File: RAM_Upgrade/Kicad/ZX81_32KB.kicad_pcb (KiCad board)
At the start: 2 copper layers, 23 x 44 mm, 3 parts, among them IC1 CY62256NLL-55SNXI, J3 Conn_01x04_Pin, J4 828-AG11D-LF

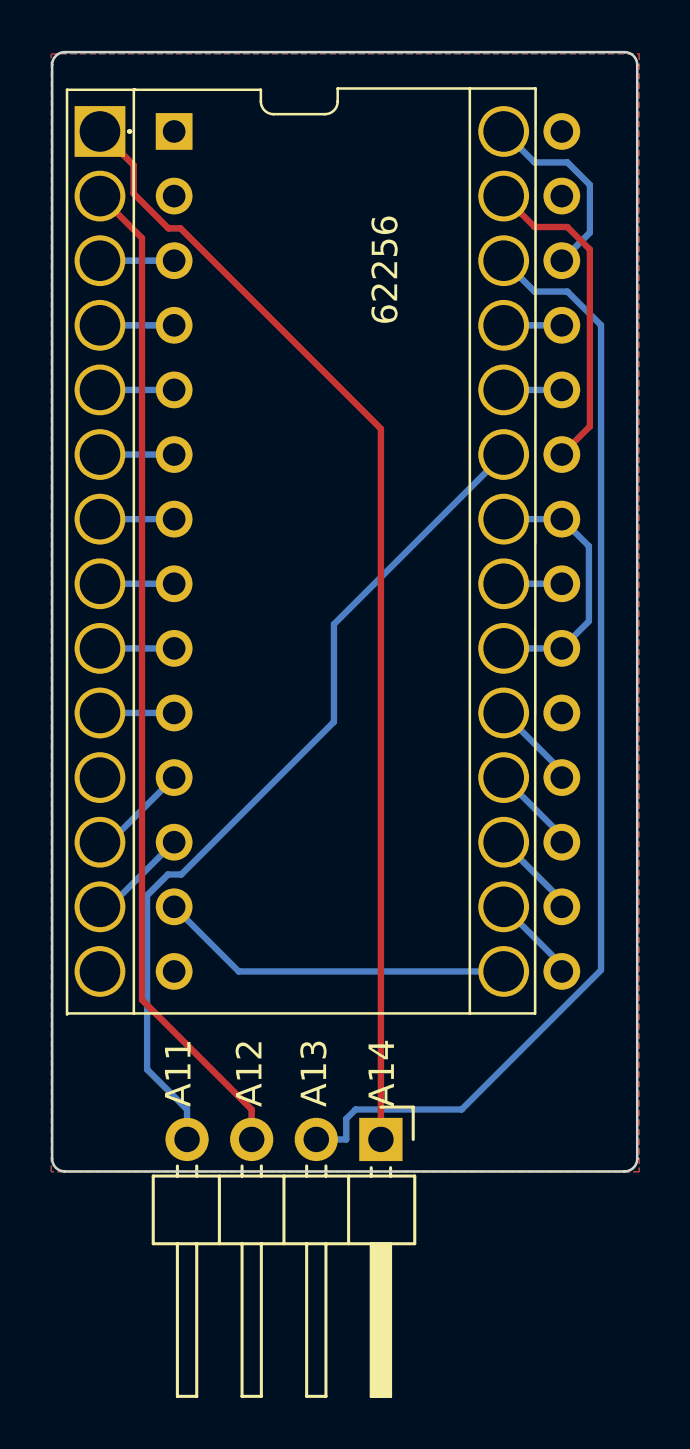
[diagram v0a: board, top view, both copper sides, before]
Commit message: Revert to original design
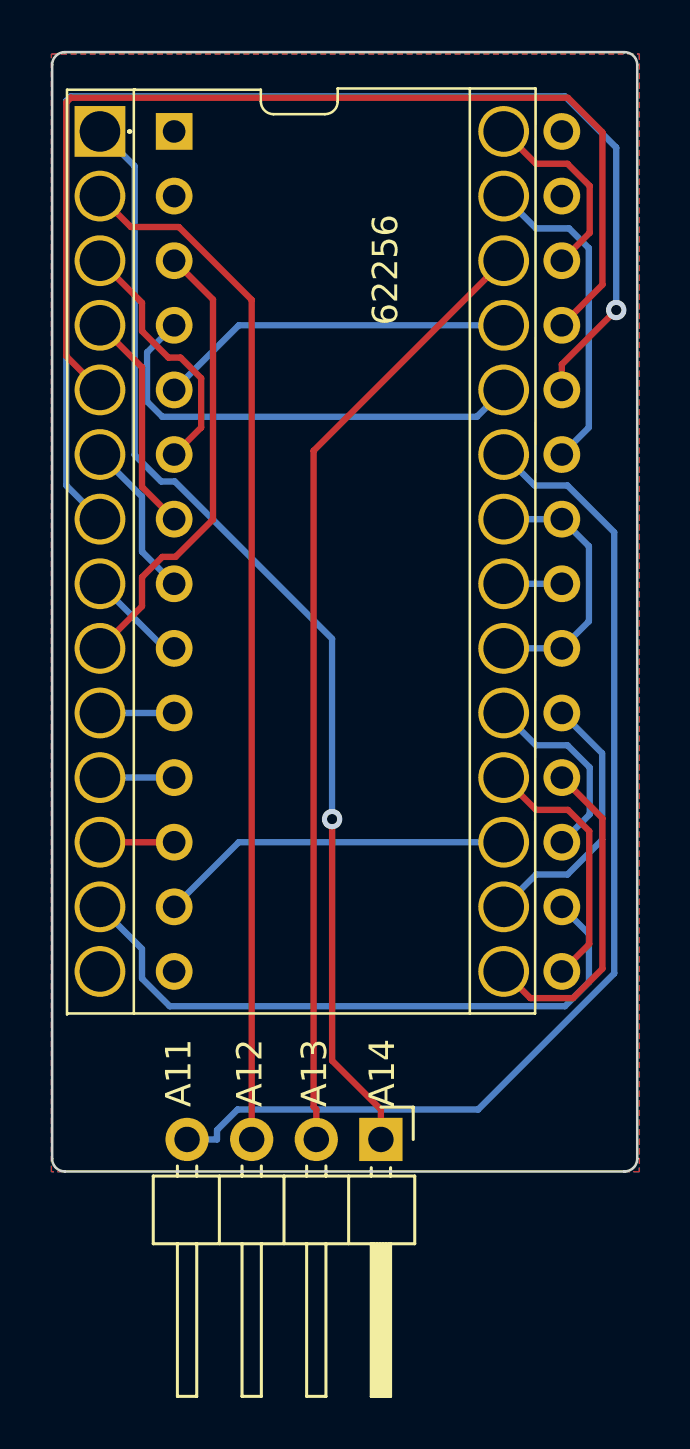
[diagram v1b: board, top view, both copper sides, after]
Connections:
- J4 pad 11: /D1 -> /D0
- J4 pad 12: /D2 -> /D1
- J4 pad 13: /D3 -> /D5
- J4 pad 15: /D4 -> /D6
- J4 pad 16: /D5 -> /D2
- J4 pad 17: /D6 -> /D7
- J4 pad 18: /D7 -> /D3
- J4 pad 19: /D8 -> /D4
- J4 pad 24: /A09 -> /A03
- J4 pad 25: /A08 -> /A05
- J4 pad 3: /A07 -> /A01
- J4 pad 4: /A06 -> /A09
- J4 pad 5: /A05 -> /A08
- J4 pad 6: /A04 -> /A07
- J4 pad 7: /A03 -> /A06
- J4 pad 8: /A02 -> /A04
- J4 pad 9: /A01 -> /A02
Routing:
- net /A03: track 2.92 -> 49.9 mm, vias 0 -> 1
- net /A05: track 2.92 -> 41.8 mm
- net /D2: track 3.97 -> 25.3 mm
- net /A09: track 2.29 -> 18.1 mm
- net /A01: track 2.92 -> 18.0 mm
- net /A08: track 2.29 -> 14.0 mm
- net /D5: track 3.49 -> 14.0 mm
- net /A11: track 33.7 -> 42.7 mm
- net /D4: track 3.49 -> 10.6 mm
- net /A07: track 2.92 -> 9.99 mm
- net /A13: track 44.7 -> 37.7 mm
- net /D6: track 3.49 -> 10.2 mm
- net /A06: track 2.92 -> 8.83 mm
- net /D7: track 3.49 -> 7.66 mm
- net /A04: track 2.92 -> 6.29 mm
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
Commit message: Corrected initial version
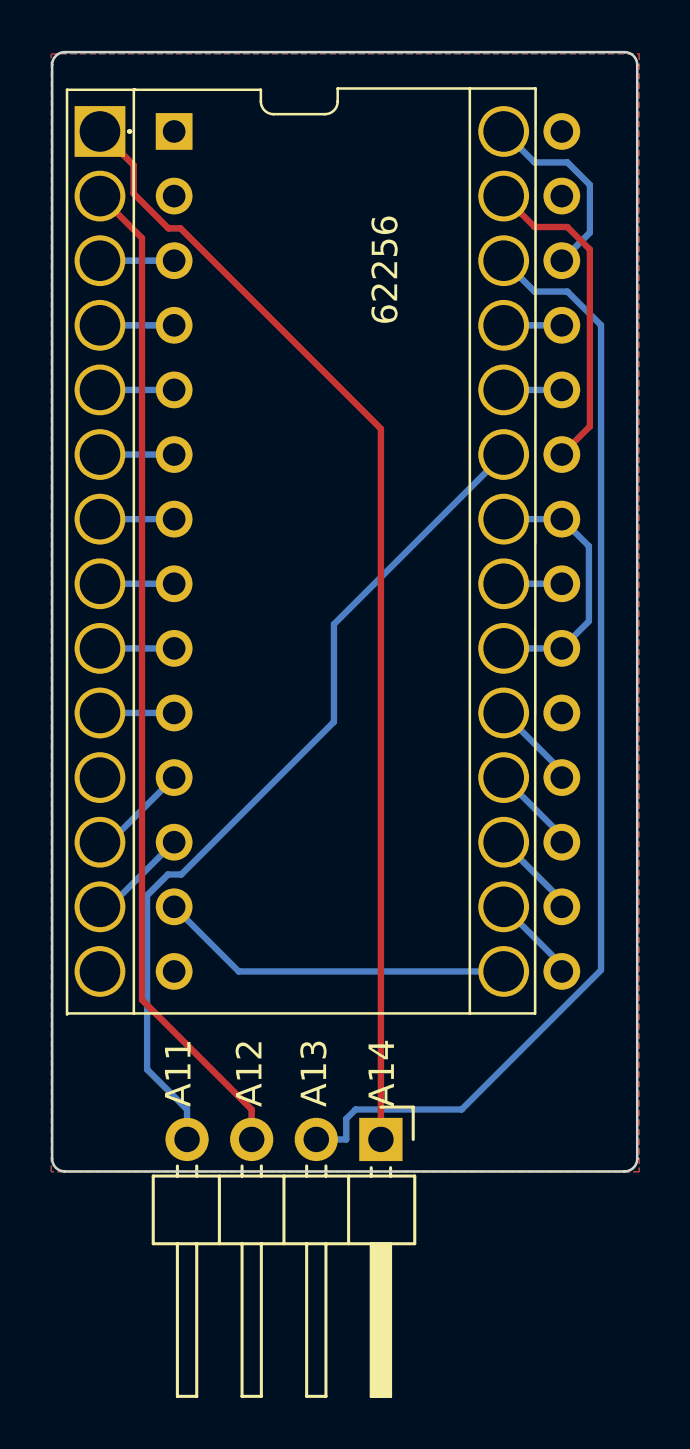
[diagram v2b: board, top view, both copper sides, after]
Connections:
- J4 pad 11: /D0 -> /D1
- J4 pad 12: /D1 -> /D2
- J4 pad 13: /D5 -> /D3
- J4 pad 15: /D6 -> /D4
- J4 pad 16: /D2 -> /D5
- J4 pad 17: /D7 -> /D6
- J4 pad 18: /D3 -> /D7
- J4 pad 19: /D4 -> /D8
- J4 pad 24: /A03 -> /A09
- J4 pad 25: /A05 -> /A08
- J4 pad 3: /A01 -> /A07
- J4 pad 4: /A09 -> /A06
- J4 pad 5: /A08 -> /A05
- J4 pad 6: /A07 -> /A04
- J4 pad 7: /A06 -> /A03
- J4 pad 8: /A04 -> /A02
- J4 pad 9: /A02 -> /A01
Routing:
- net /A03: track 49.9 -> 2.92 mm, vias 1 -> 0
- net /A05: track 41.8 -> 2.92 mm
- net /D2: track 25.3 -> 3.97 mm
- net /A09: track 18.1 -> 2.29 mm
- net /A01: track 18.0 -> 2.92 mm
- net /A08: track 14.0 -> 2.29 mm
- net /D5: track 14.0 -> 3.49 mm
- net /A11: track 42.7 -> 33.7 mm
- net /D4: track 10.6 -> 3.49 mm
- net /A07: track 9.99 -> 2.92 mm
- net /A13: track 37.7 -> 44.7 mm
- net /D6: track 10.2 -> 3.49 mm
- net /A06: track 8.83 -> 2.92 mm
- net /D7: track 7.66 -> 3.49 mm
- net /A04: track 6.29 -> 2.92 mm
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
